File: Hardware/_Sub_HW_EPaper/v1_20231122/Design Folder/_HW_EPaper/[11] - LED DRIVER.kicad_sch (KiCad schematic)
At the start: 4 parts, among them J1101 HDR_2POS_VERT, J1102 HDR_2POS_VERT

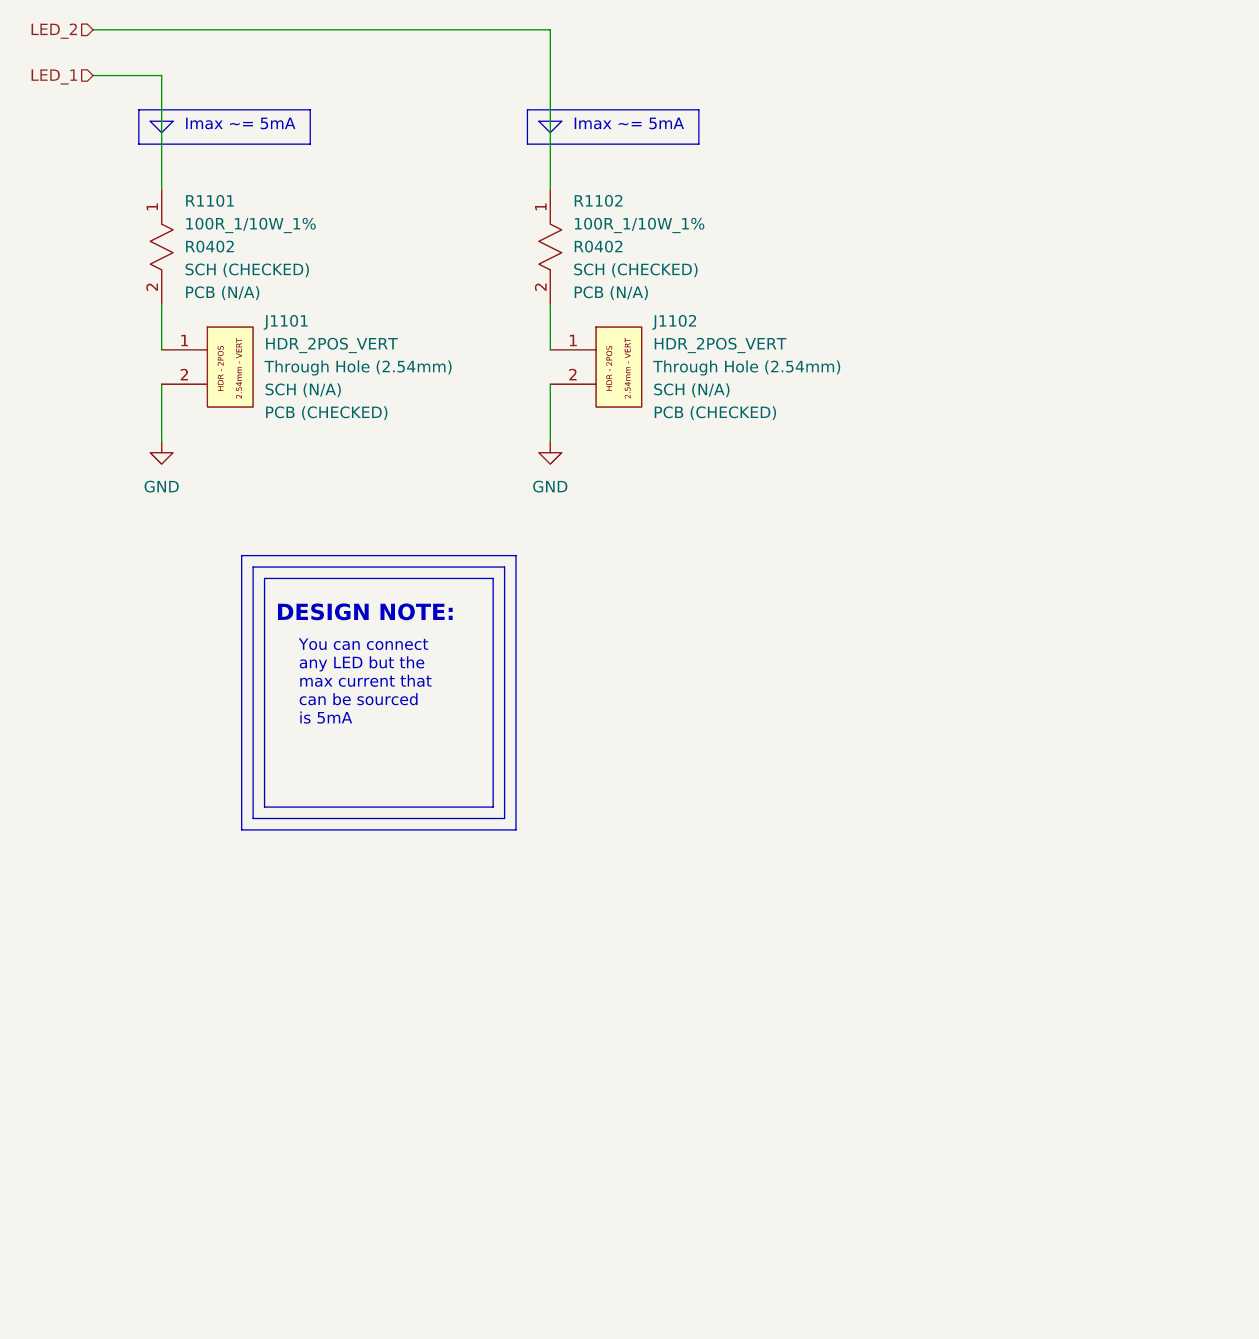
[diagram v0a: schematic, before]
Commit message: Updating file templates and structures...
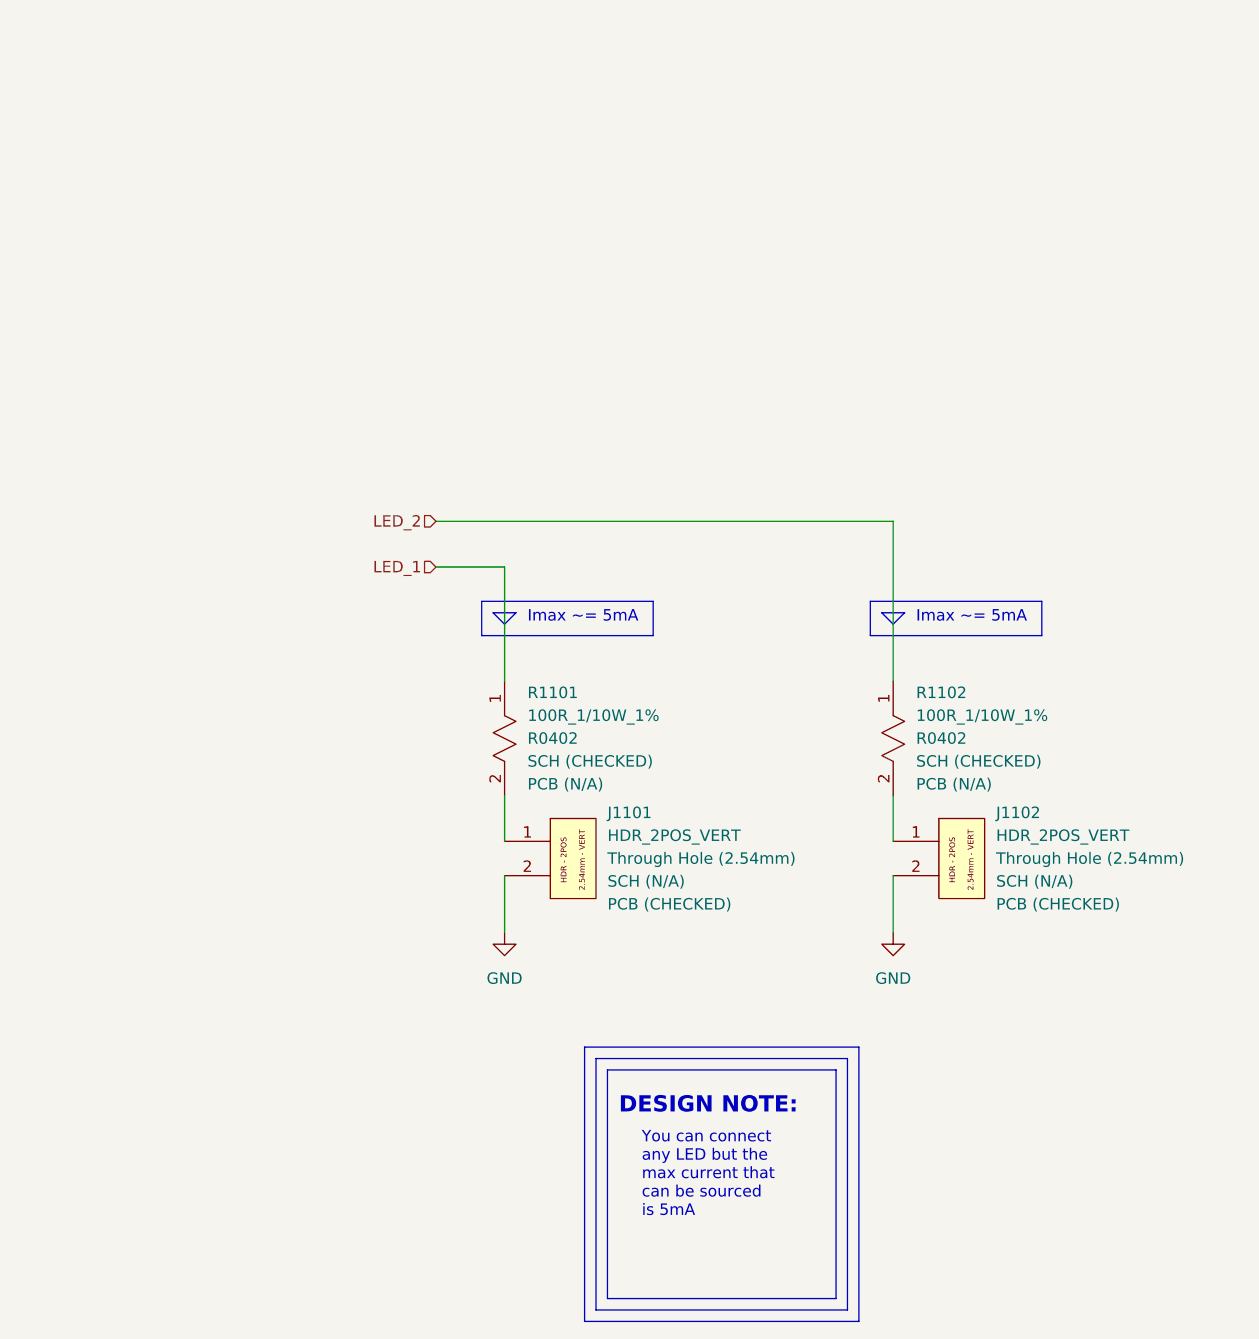
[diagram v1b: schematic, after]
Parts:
- J1101, J1102: Manufacturer (none) -> Adam Tech; Part Number PH1-02-UA -> (none); Part Number (Manufacturer) (none) -> PH1-02-UA; Part Number (Vendor) (none) -> 2057-PH1-02-UA-ND; Vendor (none) -> Digikey
- R1101, R1102: Manufacturer (none) -> KOA Speer Electronics, Inc.; Part Number RK73H1ETTP1000F -> (none); Part Number (Manufacturer) (none) -> RK73H1ETTP1000F; Part Number (Vendor) (none) -> 2019-RK73H1ETTP1000FTR-ND; Vendor (none) -> Digikey
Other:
- moved on the sheet: J1101, J1102, R1101, R1102
